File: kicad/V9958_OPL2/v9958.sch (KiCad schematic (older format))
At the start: 50 parts, among them P1 RED, P2 GREEN, P3 BLUE, P4 SYNC/C, U1 74LS139, U2 V9958, U3 DRAM_64KX4, U4 DRAM_64KX4, U5 DRAM_64KX4, U6 DRAM_64KX4, U7 cxa2075M, U8 YM3812, X1 OSC, X2 S-VIDEO, Y1 21,443Mhz

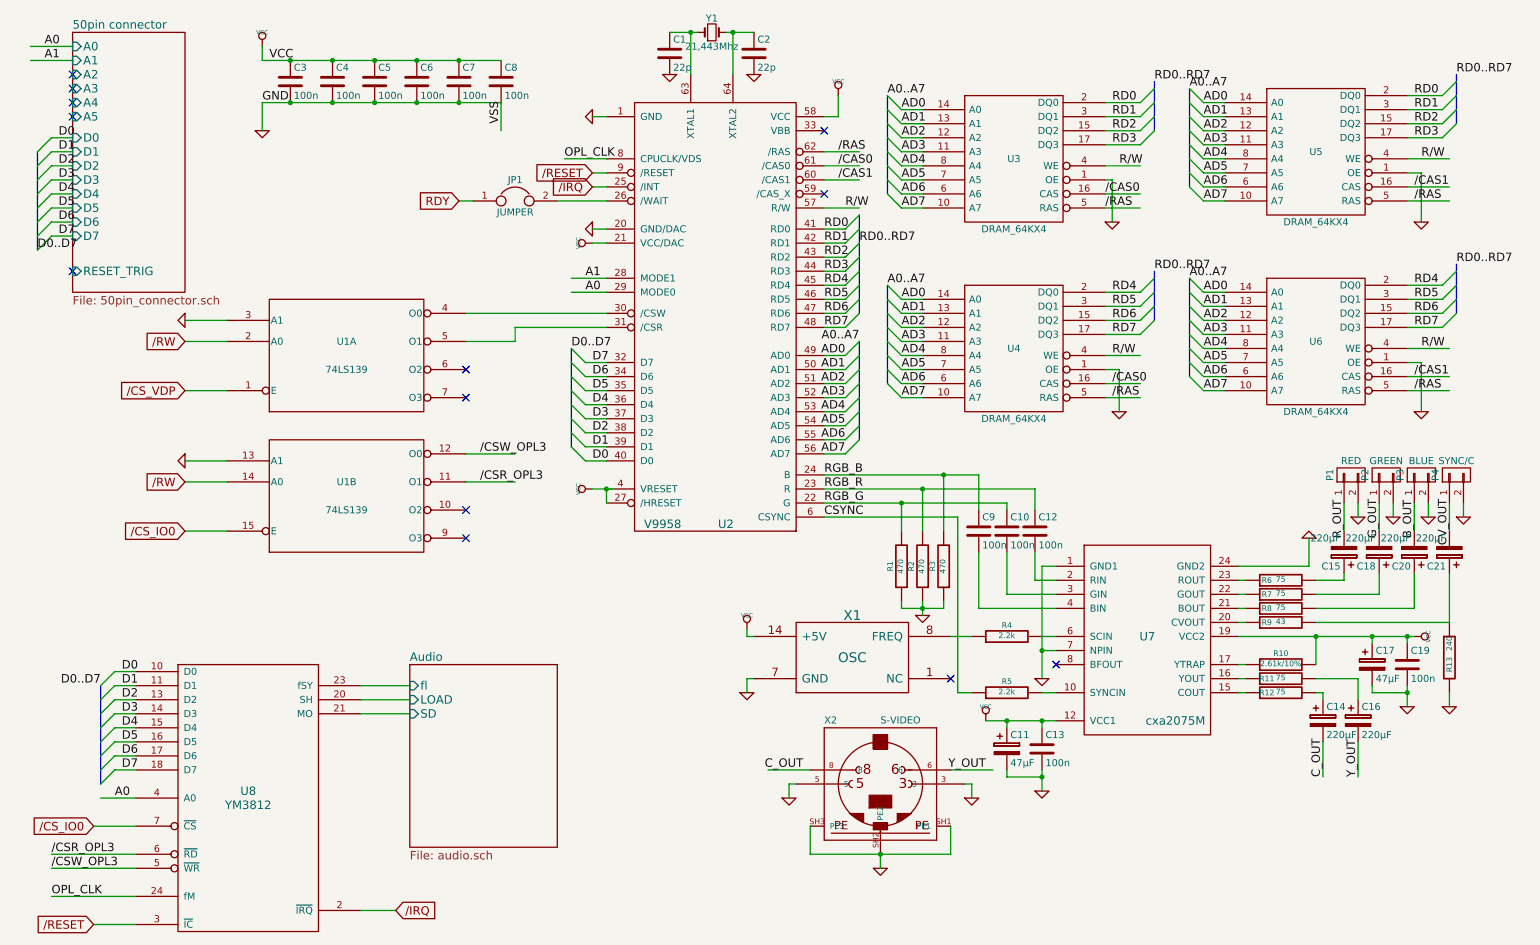
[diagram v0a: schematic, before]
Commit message: ext mem
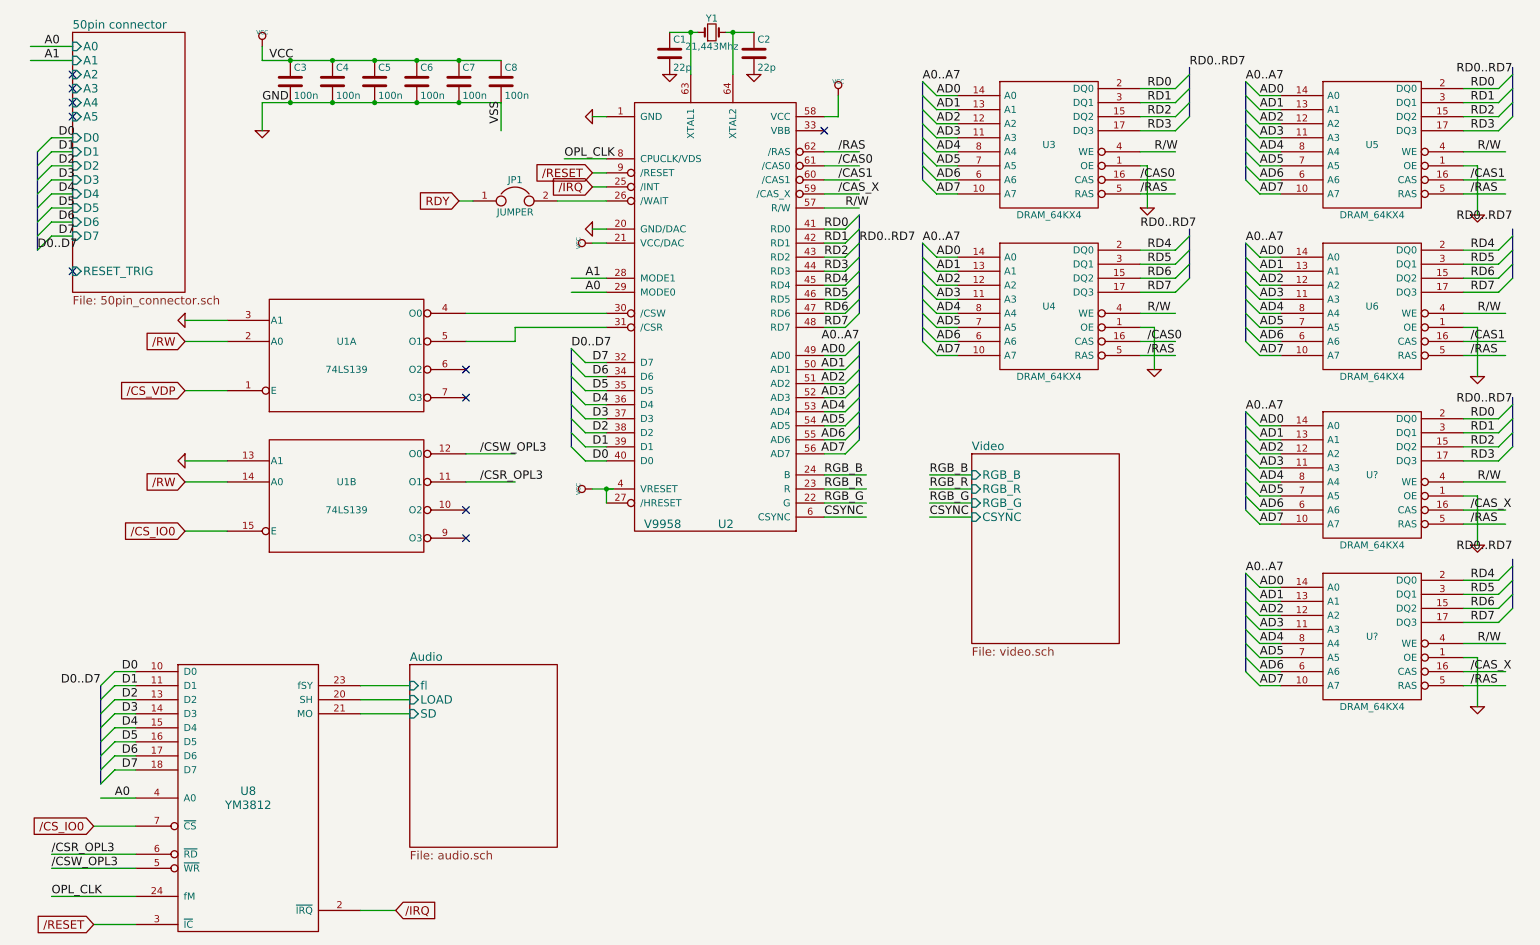
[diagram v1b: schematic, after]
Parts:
- removed C10, C12, C13, C19, C9: 100n, Capacitors_ThroughHole:C_Disc_D3_P2.5, symbol C
- removed C11, C17: 47µF, Capacitors_ThroughHole:C_Radial_D5_L11_P2.5, symbol CP
- removed C14, C15, C16, C18, C20, C21: 220µF, Capacitors_ThroughHole:C_Radial_D6.3_L11.2_P2.5, symbol CP
- removed P1: RED, w_conn_av:rca_black, symbol CONN_01X02
- removed P2: GREEN, w_conn_av:rca_black, symbol CONN_01X02
- removed P3: BLUE, w_conn_av:rca_black, symbol CONN_01X02
- removed P4: SYNC/C, w_conn_av:rca_black, symbol CONN_01X02
- removed R1, R2, R3: 470, Discret:R3, symbol R-RESCUE-v9958
- removed R10: 2.61k/10%, Discret:R3, symbol R-RESCUE-v9958
- removed R11, R12, R6, R7, R8: 75, Discret:R3, symbol R-RESCUE-v9958
- removed R13: 240, Discret:R3, symbol R-RESCUE-v9958
- removed R4, R5: 2.2k, Discret:R3, symbol R-RESCUE-v9958
- removed R9: 43, Discret:R3, symbol R-RESCUE-v9958
- removed U7: cxa2075M, Housings_SOIC:SOIC-24_7.5x15.4mm_Pitch1.27mm, symbol cxa2075M
- removed X1: OSC, Oscillators:KXO-200_LargePads, symbol OSC
- removed X2: S-VIDEO, mini_din:mini_din-M_DIN4, symbol MINI_DIN_4
- added U? (x2): DRAM_64KX4, Housings_DIP:DIP-18_W7.62mm_LongPads, symbol DRAM_64KX4
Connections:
- net labels added: /CAS_X
- net labels removed: B_OUT, CV_OUT, C_OUT, G_OUT, R_OUT, Y_OUT
- wire segments 247 -> 202
- no-connect marks 13 -> 10
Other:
- moved on the sheet: U3, U4, U5, U6
